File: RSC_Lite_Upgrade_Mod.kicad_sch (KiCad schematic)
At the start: 23 parts, among them J1 USB_B_Micro, J2 Boot Mode, J3 SWD, SW1 RESET, U1 STM32F103C8Tx, Y1 8Mhz

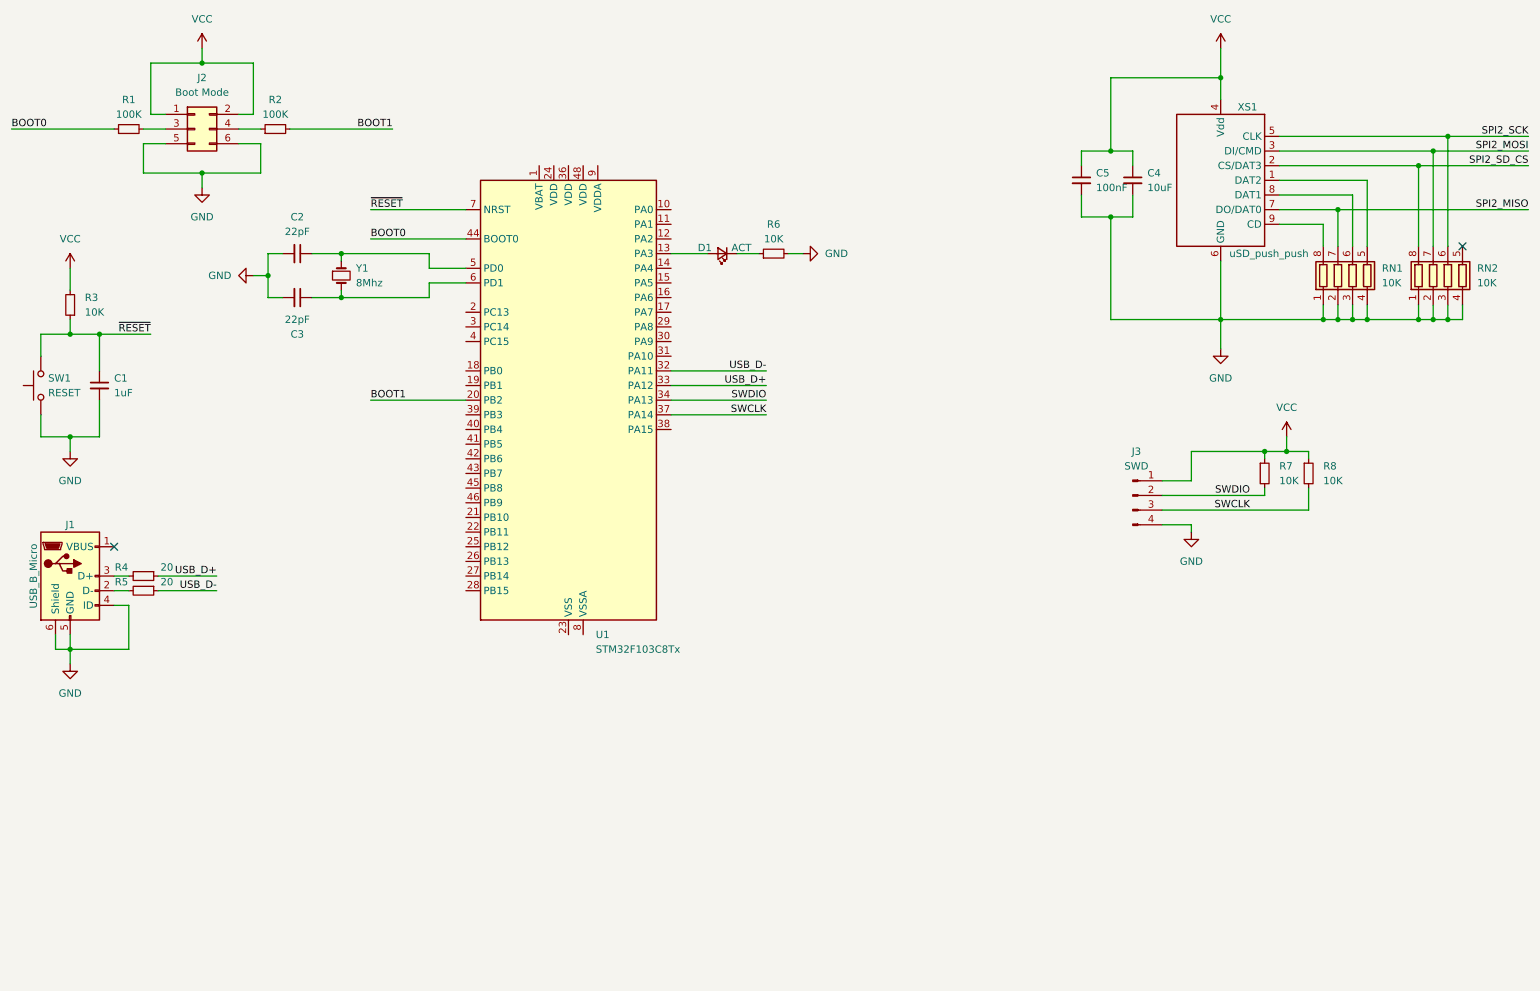
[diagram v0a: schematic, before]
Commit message: Update schematics
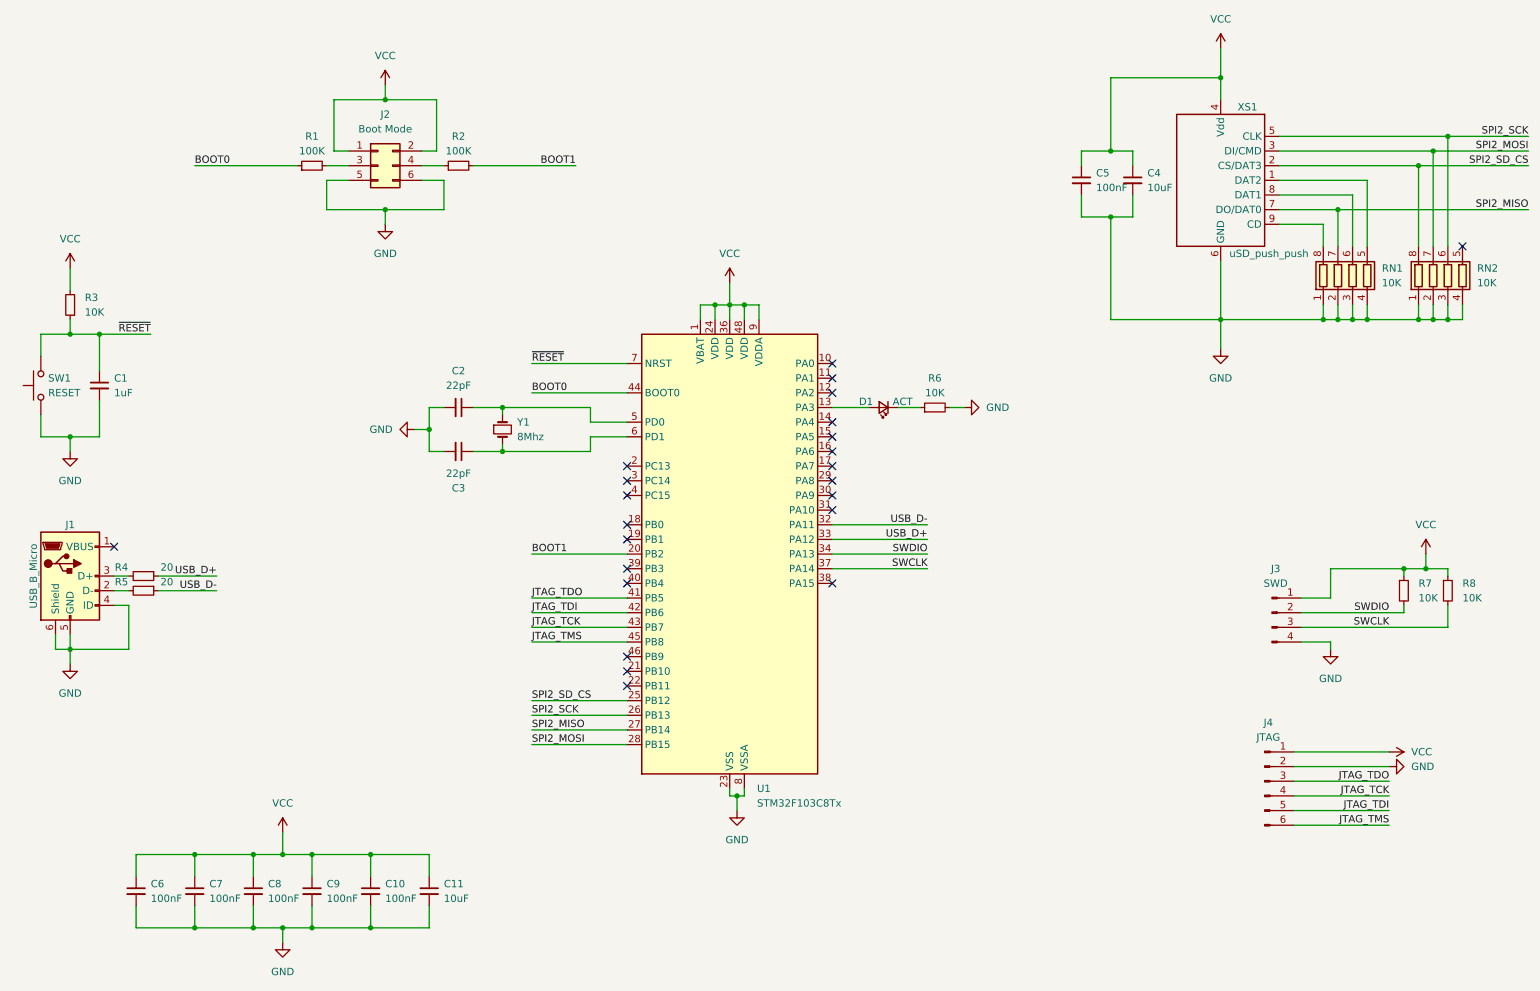
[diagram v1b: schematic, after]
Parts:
- added C10, C6, C7, C8, C9: 100nF, symbol Device:C_Small
- added C11: 10uF, symbol Device:C_Small
- added J4: JTAG, symbol Connector:Conn_01x06_Pin
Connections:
- net GND: now also U1.23 (VSS), U1.35 (VSS), U1.47 (VSS), U1.8 (VSSA), C10.2, C11.2, C6.2, C7.2, C8.2, C9.2, J4.2 (Pin_2)
- net SPI2_MISO: now also U1.27 (PB14)
- net SPI2_MOSI: now also U1.28 (PB15)
- net SPI2_SCK: now also U1.26 (PB13)
- net SPI2_SD_CS: now also U1.25 (PB12)
- net VCC: now also U1.1 (VBAT), U1.24 (VDD), U1.36 (VDD), U1.48 (VDD), U1.9 (VDDA), C10.1, C11.1, C6.1, C7.1, C8.1, C9.1, J4.1 (Pin_1)
- net JTAG_TDO: now reaches U1.41 (PB5)
- net JTAG_TDO: now also J4.3 (Pin_3)
- net JTAG_TDI: now reaches U1.42 (PB6)
- net JTAG_TDI: now also J4.5 (Pin_5)
- net JTAG_TCK: now reaches U1.43 (PB7)
- net JTAG_TCK: now also J4.4 (Pin_4)
- net JTAG_TMS: now reaches U1.45 (PB8)
- net JTAG_TMS: now also J4.6 (Pin_6)
- no-connect marks 2 -> 23
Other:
- moved on the sheet: C2, C3, D1, J2, J3, R1, R2, R6, R7, R8, U1, Y1
